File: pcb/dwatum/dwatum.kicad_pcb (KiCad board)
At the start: 4 copper layers, 37.5 x 17.5 mm, 39 parts, among them J1 TC2030-CC2538-BL, P1 CONN_01X02, U1 DWM1000, U2 CC2538, U3 TPS727xx, U4 TPS62740, X1 CRYSTAL_SMD_4, Y1 Crystal

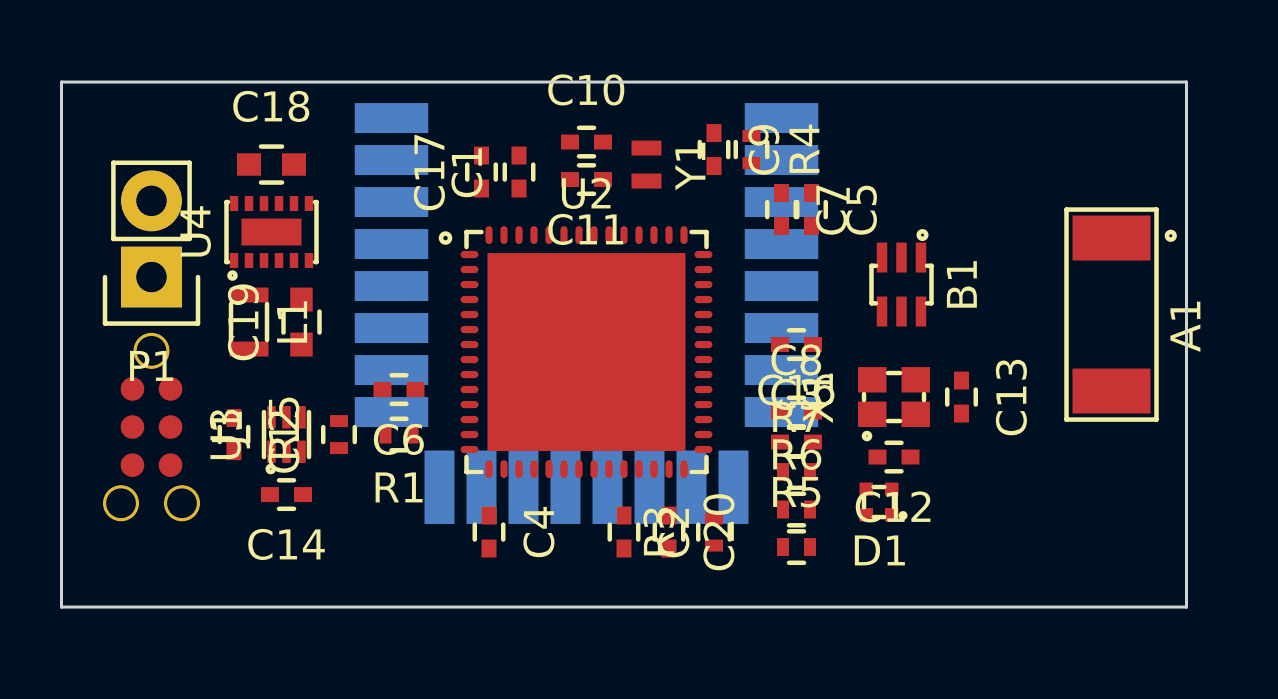
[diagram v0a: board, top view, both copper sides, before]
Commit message: most of the routing is done with dwatum
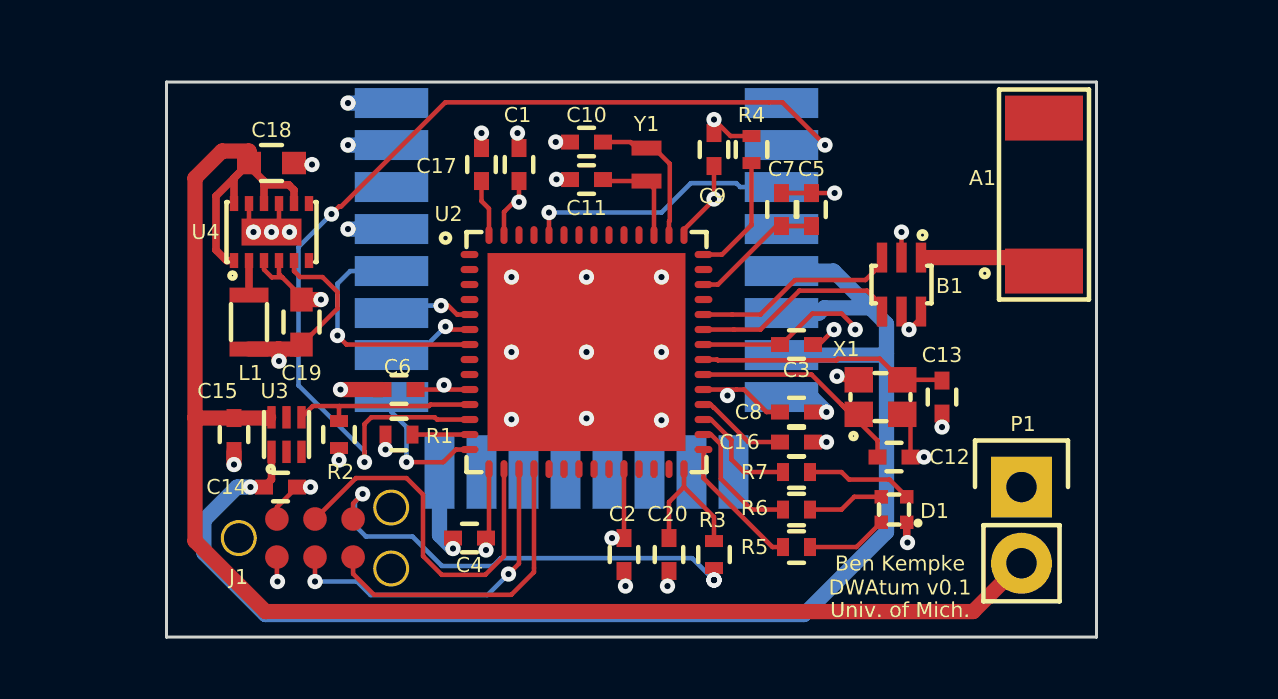
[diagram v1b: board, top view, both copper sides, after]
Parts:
- moved P1 29.8 mm to (188.5, 86.0), turned to 0 degrees
- moved J1 6.59 mm to (164.9, 87.7), turned to 0 degrees
- moved A1 4.59 mm to (189.2, 76.2), turned to 90 degrees
- moved C2 0.75 mm to (175.2, 88.2)
- moved C20 0.75 mm to (176.8, 88.2)
- moved R3 0.75 mm to (178.2, 88.2)
- moved C4 0.68 mm to (170.1, 87.7), turned to 180 degrees
- moved C13 0.65 mm to (185.8, 83.0)
- moved D1 0.56 mm to (184.2, 86.8)
- moved U1 0.50 mm to (174.0, 85.5)
- moved X1 0.45 mm to (183.8, 83.0)
- moved C14 0.32 mm to (163.8, 86.0), turned to 0 degrees
- moved C1 0.25 mm to (171.8, 75.2)
- moved C17 0.25 mm to (170.5, 75.2)
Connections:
- U1 pad 5: VCC -> VAA
- U1 pad 6: VCC -> VAA
- U1 pad 7: VCC -> VAA
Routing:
- net +BATT: track 0.00 -> 56.3 mm
- net VAA: track 0.00 -> 47.3 mm, vias 0 -> 1
- net GND: track 0.00 -> 40.1 mm, vias 0 -> 39
- net DW_WAKEUP: track 0.00 -> 34.6 mm, vias 0 -> 3
- net VCC: track 0.00 -> 33.5 mm, vias 0 -> 10
- net ~RESET: track 0.00 -> 15.1 mm, vias 0 -> 3
- net BOOTLOADER_RX: track 0.00 -> 12.6 mm
- net BOOTLOADER_TX: track 0.00 -> 11.4 mm, vias 0 -> 2
- net BOOTLOADER_CTRL: track 0.00 -> 10.6 mm
- net DW_RSTn: track 0.00 -> 8.96 mm, vias 0 -> 1
- net Net-(C13-Pad1): track 0.00 -> 8.28 mm
- net SPI_SCK: track 0.00 -> 8.23 mm, vias 0 -> 1
- net Net-(C12-Pad2): track 0.00 -> 7.96 mm
- net Net-(B1-Pad4): track 0.00 -> 6.89 mm
- net Net-(B1-Pad3): track 0.00 -> 6.85 mm
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- added copper zone on In1.Cu, net GND
- added copper zone on In2.Cu, net VCC
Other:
- board size 37.5 x 17.5 mm -> 31 x 18.5 mm
- rule trace_min: 0.2 -> 0.1524
- rule via_min_drill: 0.3 -> 0.2032
- rule via_min_size: 0.4 -> 0.508
- board text added: "Ben Kempke"
- board text added: "DW1000"
- board text added: "DWAtum v0.1"
- board text added: "Univ. of Mich."
